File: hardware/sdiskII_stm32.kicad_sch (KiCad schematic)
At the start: 28 parts, among them J1 PWR, J2 APPLE_SDISKII, J3 Conn_01x06, J4 UART, J5 Conn_01x04, J6 STLINK, J7 PWR, U1 LM1117MP-3.3, U2 MicroSD_SDIO, U8 DM-OLED096-636

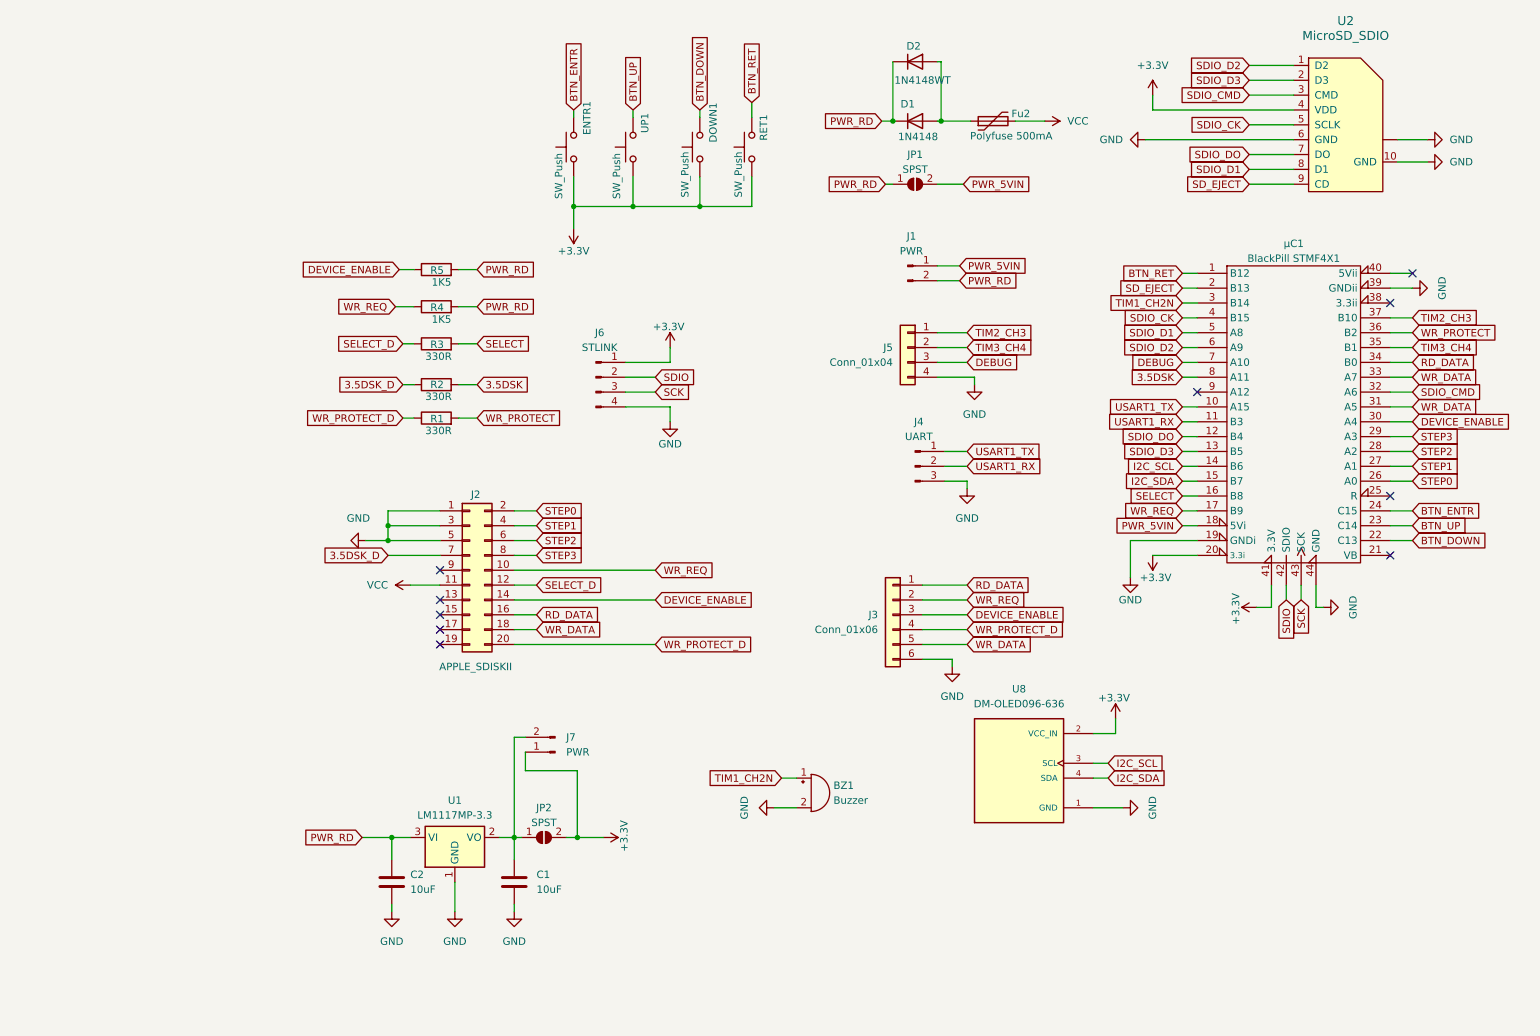
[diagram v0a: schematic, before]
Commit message: v0.80.17 Alpha
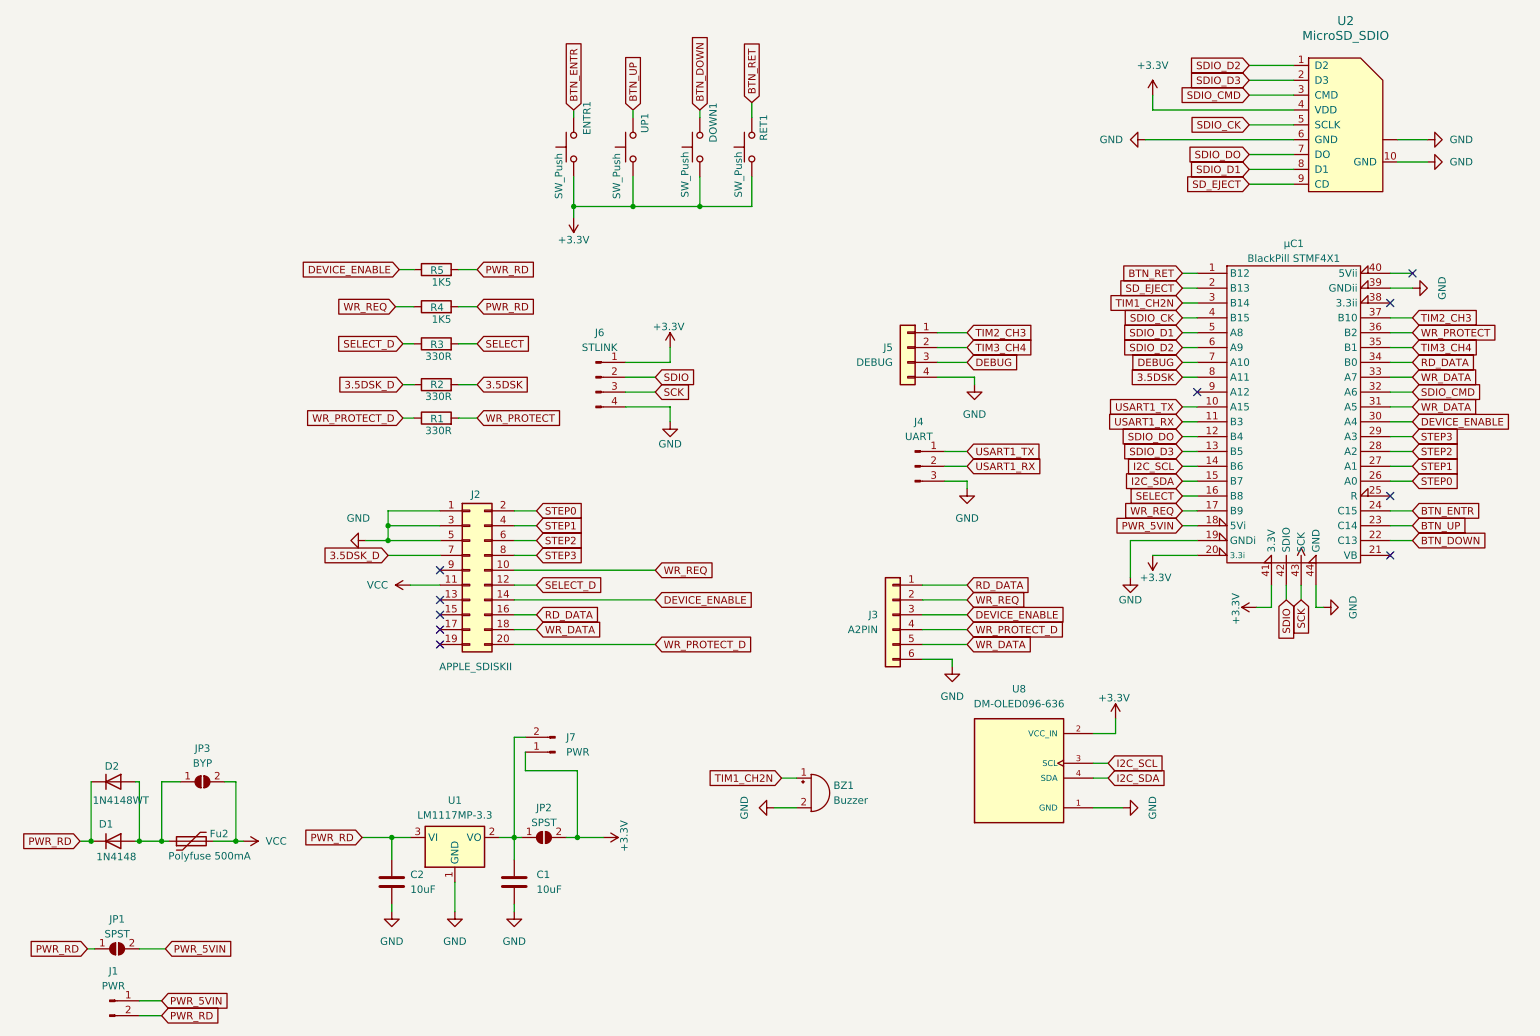
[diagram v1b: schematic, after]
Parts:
- added JP3: BYP, Jumper:SolderJumper-2_P1.3mm_Open_RoundedPad1.0x1.5mm, symbol Jumper:SolderJumper_2_Open
- J3: value Conn_01x06 -> A2PIN
- J5: value Conn_01x04 -> DEBUG
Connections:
- net VCC: now also JP3.2 (B)
- net at D1.2 (A), D2.2 (A), Fu2.1: now also JP3.1 (A)
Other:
- moved on the sheet: D1, D2, Fu2, J1, JP1
